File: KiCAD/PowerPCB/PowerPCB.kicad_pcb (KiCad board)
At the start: 2 copper layers, 32 x 19.5 mm, 13 parts, among them J1 GPIO, J2 Power In, J5 Serial, J6 Fan, Q1 DMMT5401, Q2 IRLML6401, Q3 IRLML6344

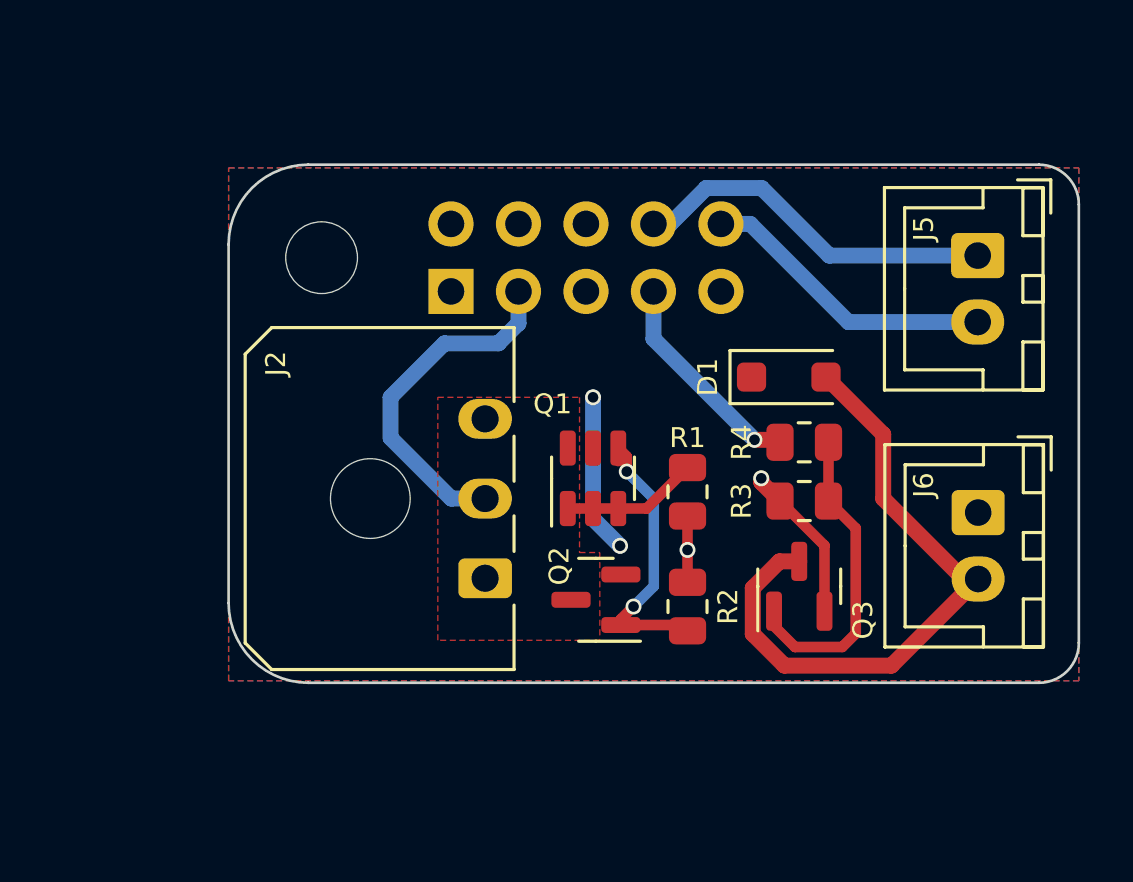
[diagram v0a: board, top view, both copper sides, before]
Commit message: Update PCBLayout
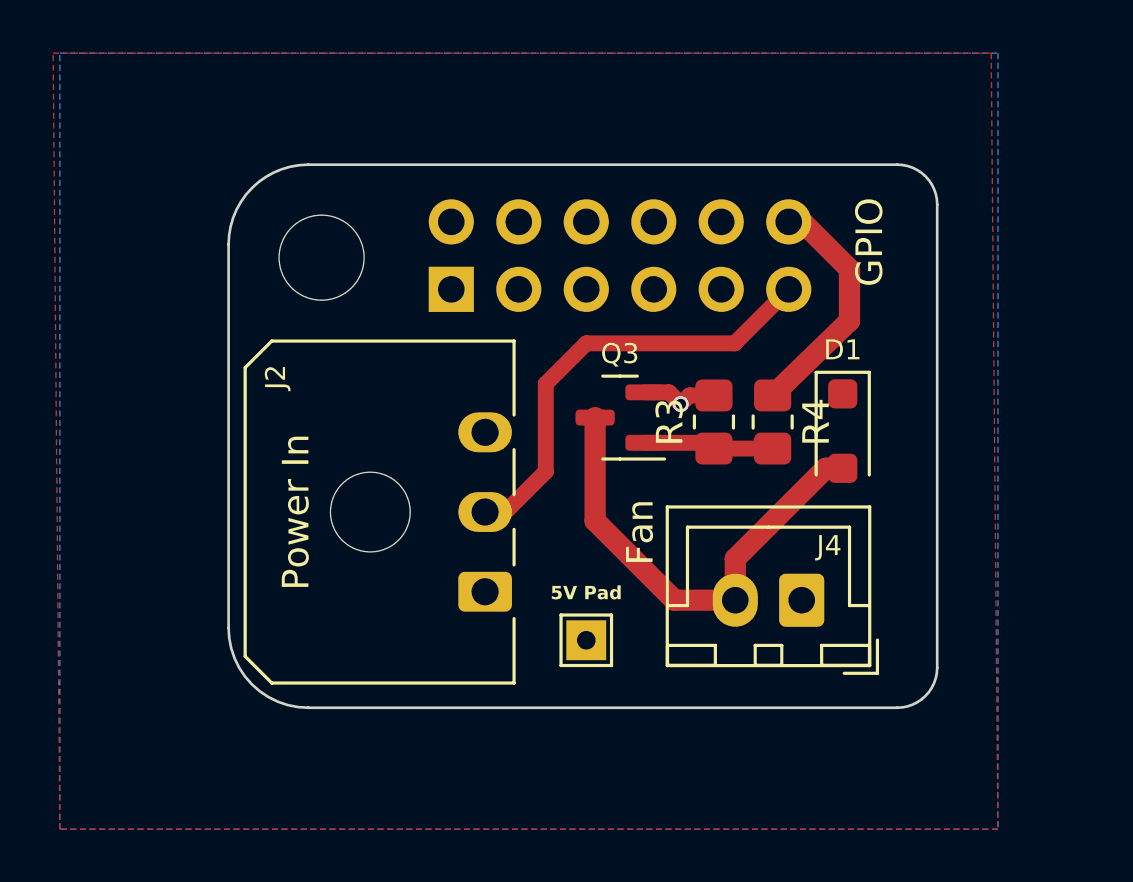
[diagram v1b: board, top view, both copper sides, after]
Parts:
- removed J5: Serial, Connector_JST:JST_XH_B2B-XH-A_1x02_P2.50mm_Vertical
- removed Q1: DMMT5401, Package_TO_SOT_SMD:SOT-23-6
- removed Q2: IRLML6401, Package_TO_SOT_SMD:SOT-23
- removed R1: 10k, Resistor_SMD:R_0805_2012Metric
- removed R2: 47k, Resistor_SMD:R_0805_2012Metric
- added J3: 5V Pad, TestPoint:TestPoint_THTPad_1.5x1.5mm_Drill0.7mm, F.Cu at (113.5, 61.9)
- J1: footprint Connector_PinSocket_2.54mm:PinSocket_2x05_P2.54mm_Vertical -> Connector_PinSocket_2.54mm:PinSocket_2x06_P2.54mm_Vertical
- R3, R4: footprint Resistor_SMD:R_0805_2012Metric -> Resistor_SMD:R_0805_2012Metric_Pad1.20x1.40mm_HandSolder
- moved Q3 9.26 mm to (114.7, 53.5), turned to 180 degrees
- moved J4 7.42 mm to (121.6, 60.4), turned to 180 degrees
- moved R3 4.52 mm to (118.3, 53.7), turned to 90 degrees
- moved D1 2.87 mm to (123.1, 54.0), turned to -90 degrees
- moved R4 1.41 mm to (120.5, 53.7), turned to -90 degrees
- moved J2 0.51 mm to (109.7, 60.1)
- moved J1 0.08 mm to (108.4, 48.7)
- renumbered J6 to J4
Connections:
- J2 pad 1: 5V_IN -> +5V
- J2 pad 2: GPIO2/SDA1 -> GPIO17
- R4 pad 1: GPIO4/GPCLK0 -> GPIO18
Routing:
- net GPIO17: track 0.00 -> 16.8 mm
- net GPIO14/TXD0: track 13.8 -> 0.00 mm
- net GPIO2/SDA1: track 13.2 -> 0.00 mm
- net GPIO15/RXD0: track 11.2 -> 0.00 mm
- net Net-(Q1B-C): track 11.1 -> 0.00 mm, vias 2 -> 0
- net GPIO18: track 0.00 -> 9.00 mm
- net GPIO4/GPCLK0: track 8.16 -> 0.00 mm, vias 1 -> 0
- net Net-(D1-A): track 24.5 -> 17.4 mm
- net Net-(Q3-G): track 11.8 -> 4.90 mm
- net +5V: track 6.01 -> 0.00 mm, vias 2 -> 0
- net GND: track 8.48 -> 3.00 mm, vias 2 -> 1
- net Net-(Q1A-B): track 5.14 -> 0.00 mm
- removed copper zone on F.Cu, net 5V_IN
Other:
- board size 32 x 19.5 mm -> 26.7 x 20.4 mm
